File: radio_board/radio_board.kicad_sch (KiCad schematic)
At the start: 107 parts, among them CN1 HX JN1.27-2X5P ZZ H4.9, Q1 2N7002K, SW2 RKB2SJG250SMTRLFS, SW3 MSK12C02, U1 FSC-BT1036C, U2 TP4057, U3 XB5352A, U4 SKB369, U5 S2B-PH-K-S(LF)(SN), U6 TLV75533PDBVR, U7 LMV321

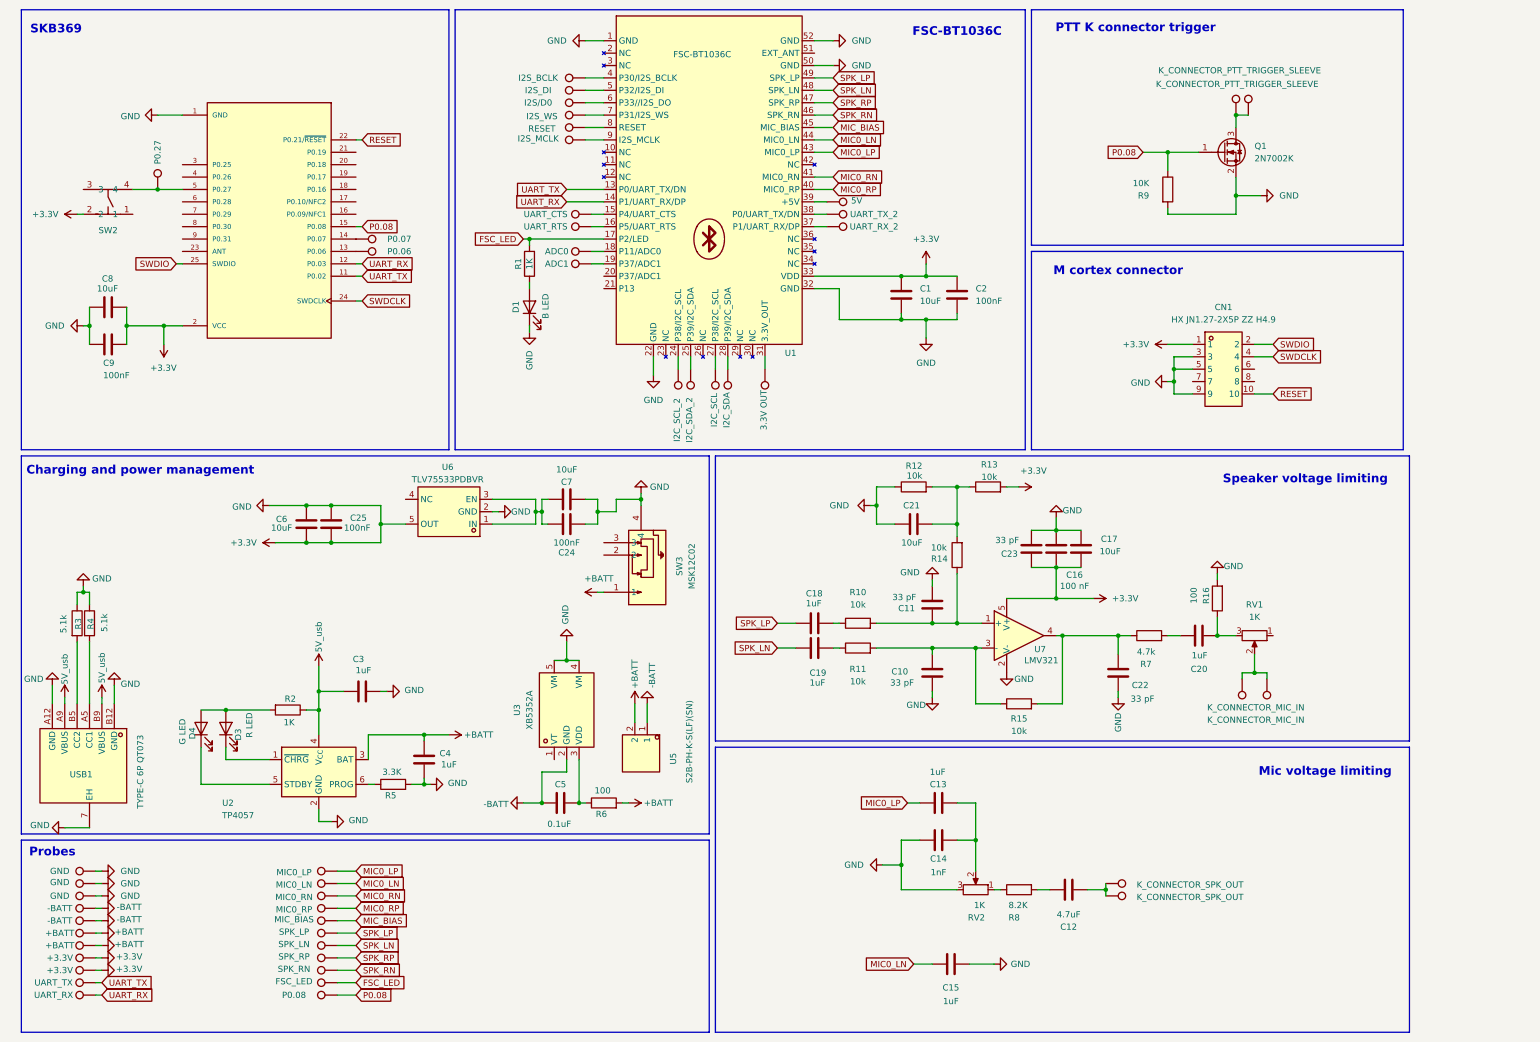
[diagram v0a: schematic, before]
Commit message: [WIP] Started net rev of ptt board and radio board
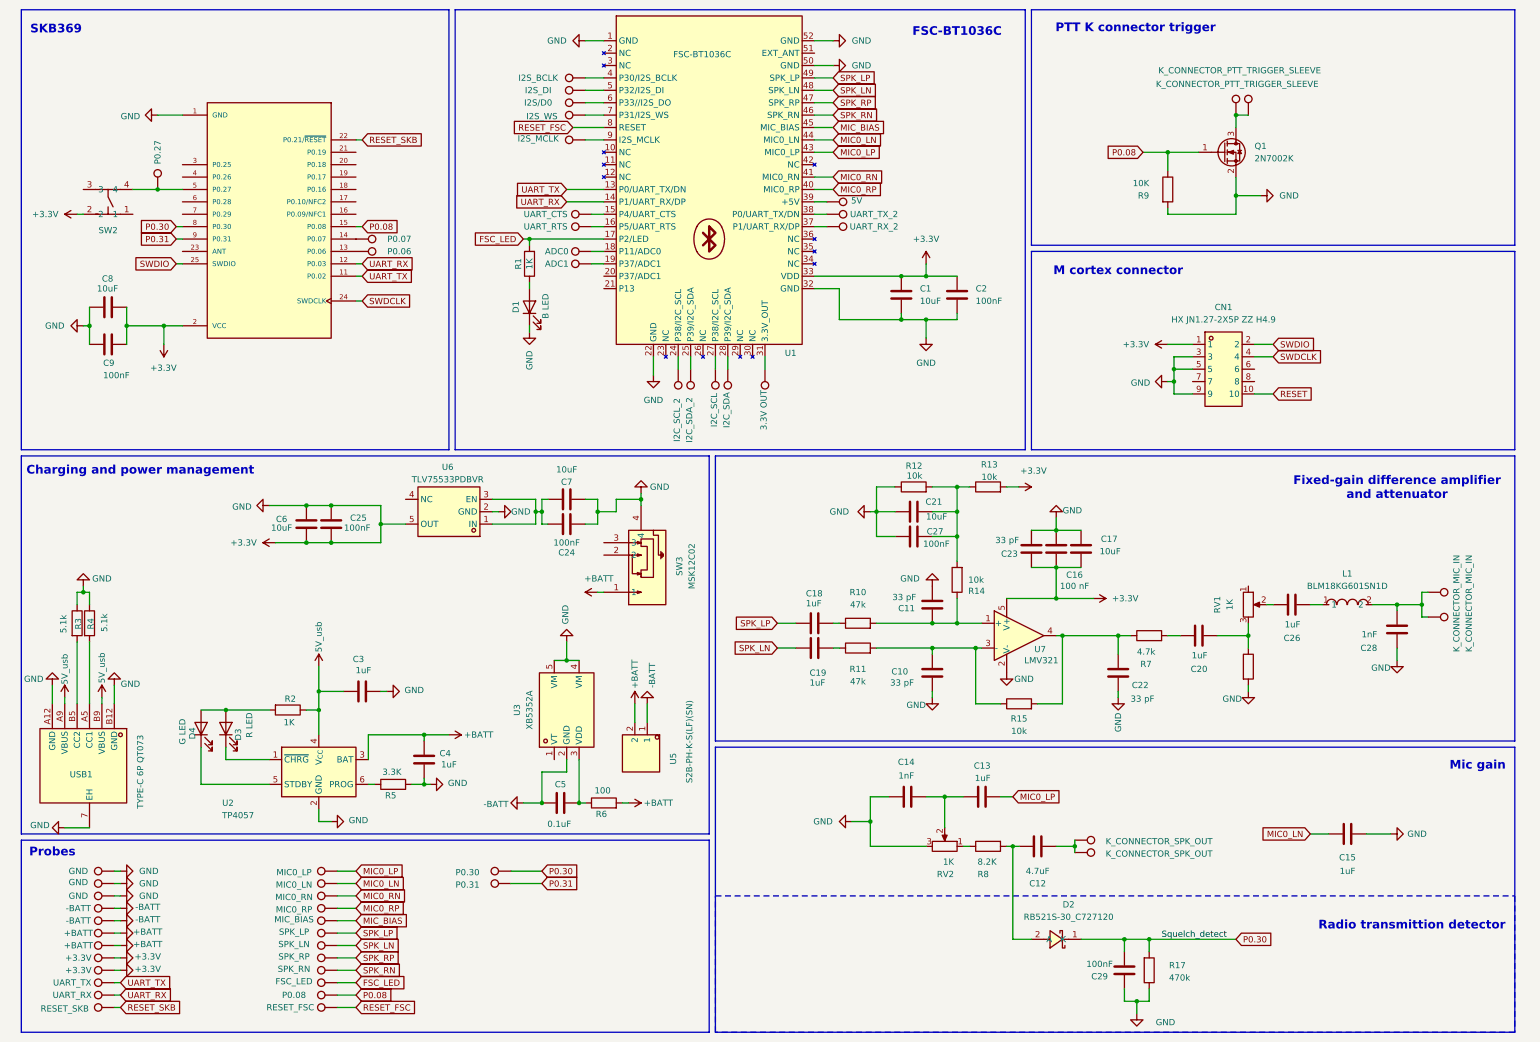
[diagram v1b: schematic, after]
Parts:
- added C26: 1uF, Resistor_SMD:R_0603_1608Metric_Pad0.98x0.95mm_HandSolder, symbol Device:C
- added C27, C29: 100nF, Resistor_SMD:R_0603_1608Metric_Pad0.98x0.95mm_HandSolder, symbol Device:C
- added C28: 1nF, Resistor_SMD:R_0603_1608Metric_Pad0.98x0.95mm_HandSolder, symbol Device:C
- added D2: RB521S-30_C727120, Project_components:SOD-523_L1.2-W0.8-LS1.6-RD, symbol PTT_project:RB521S-30_C727120
- added L1: BLM18KG601SN1D, Project_components:L0603, symbol PTT_project:BLM18KG601SN1D
- added R17: 470k, Resistor_SMD:R_0603_1608Metric_Pad0.98x0.95mm_HandSolder, symbol Device:R
- added TP37: RESET_SKB, TestPoint:TestPoint_THTPad_D2.0mm_Drill1.0mm, symbol Connector:TestPoint
- added TP44: P0.30, TestPoint:TestPoint_THTPad_D2.0mm_Drill1.0mm, symbol Connector:TestPoint
- added TP52: P0.31, TestPoint:TestPoint_THTPad_D2.0mm_Drill1.0mm, symbol Connector:TestPoint
- R10, R11: value 10k -> 47k
- TP22: value RESET -> RESET_FSC
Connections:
- net +3.3V: now also C27.1, C28.2, C29.2, R17.1
- net RESET: no longer U4.22 (P0.21/~{RESET})
- net at C12.2, R8.2: now also D2.2 (A)
- net P0.30: now reaches U4.8 (P0.30)
- net P0.30: now also C29.1, D2.1 (K), R17.2, TP44.1
- net P0.31: now reaches U4.9 (P0.31)
- net P0.31: now also TP52.1
- net at C21.2, R12.2, R13.1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: now also C27.2
- net at TP50.1, TP51.1: now also C28.1, L1.2; no longer RV1.2
- net RESET_FSC: now reaches TP22.1, U1.8 (RESET)
- new net: C26.1, RV1.2
- new net: C26.2, L1.1
- new net RESET_SKB: TP37.1, U4.22 (P0.21/~{RESET})
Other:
- note added: "Fixed-gain difference amplifier and attenuator"
- note added: "Mic gain"
- note added: "Radio transmittion detector"
- note removed: "Mic voltage limiting"
- note removed: "Speaker voltage limiting"
- moved on the sheet: C12, C13, C14, C15, C21, R14, R8, RV1, RV2
